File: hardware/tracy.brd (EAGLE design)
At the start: 58.5 x 38 mm, 78 parts, among them IC1 SIM900, J1 U.FL, J2 U.FL, Q4 si2305cd, T1 BC846, T2 BC846, U1 SPX5205 3v3, U2 3339, U3 TC1014 2V8, X1 MOLEX_6VERTICAL, X2 MOLEX_2HORIZONTAL, Y1 32768Hz CFPX-217 12.5pF

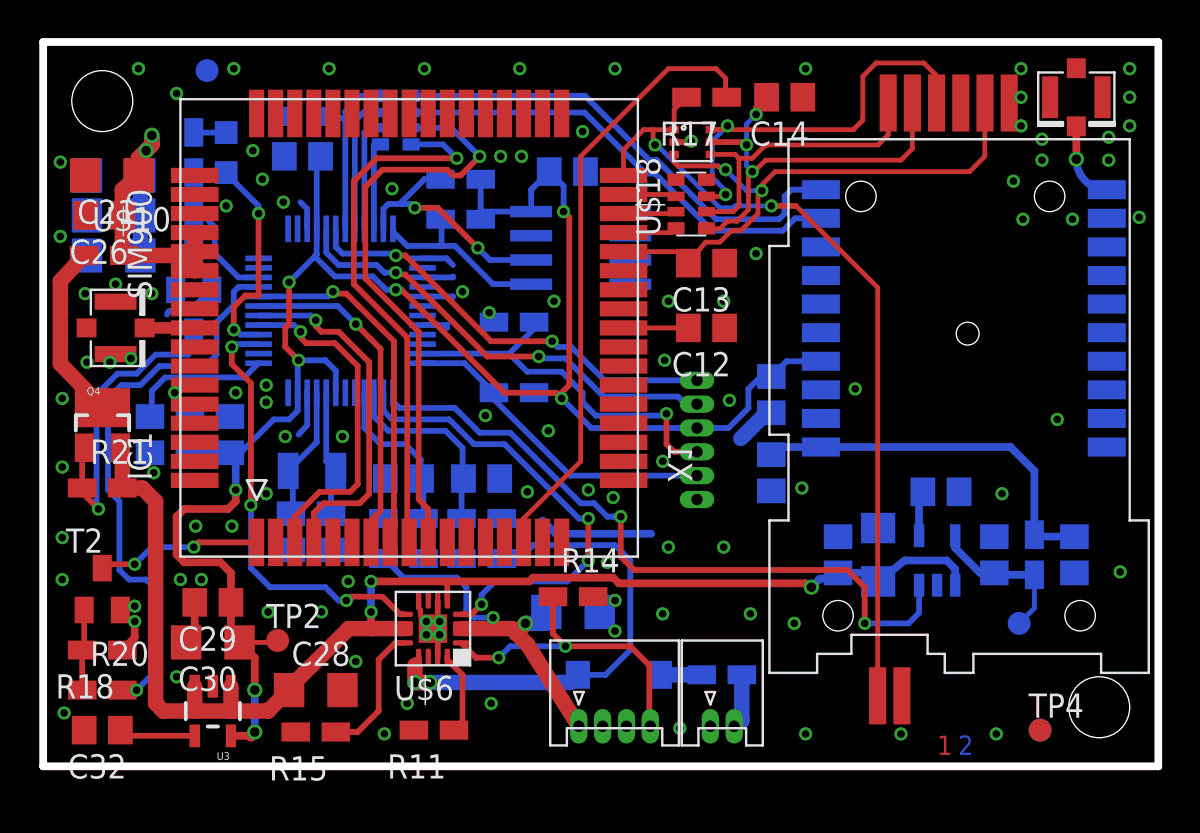
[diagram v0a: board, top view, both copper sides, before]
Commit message: rev 2
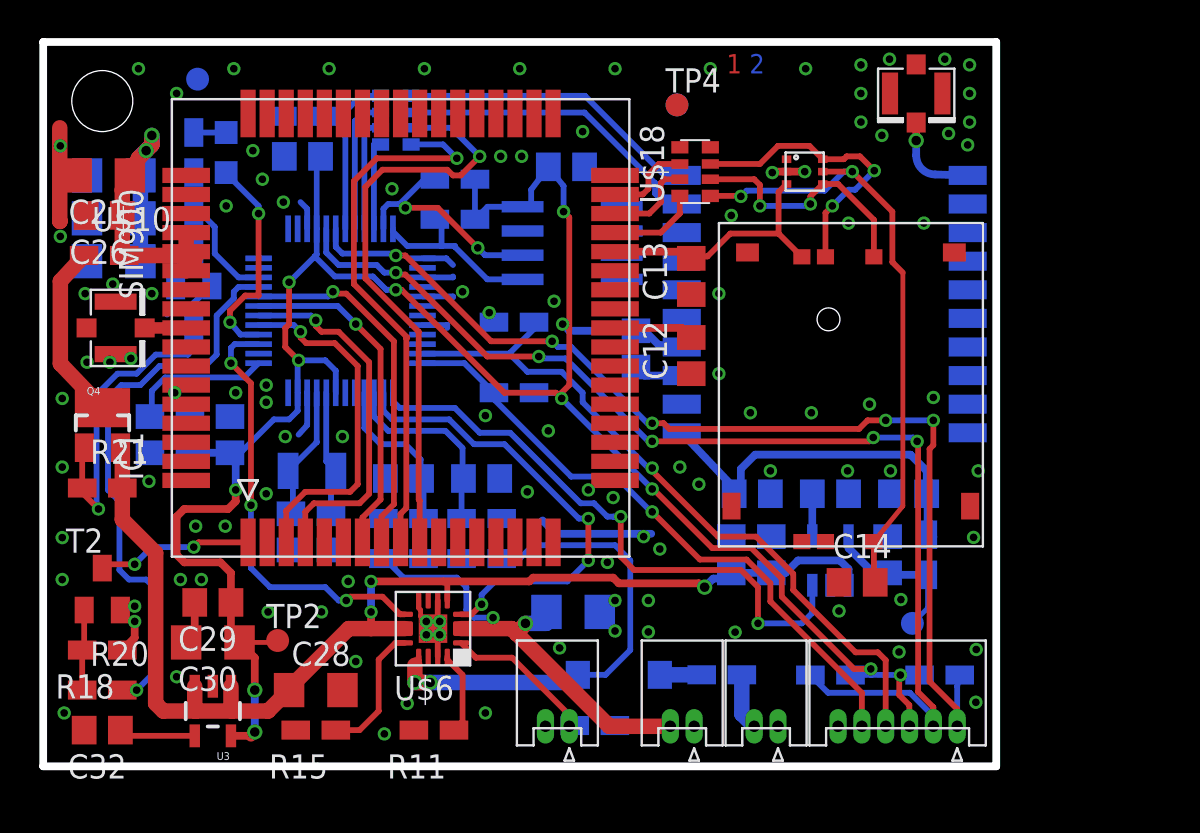
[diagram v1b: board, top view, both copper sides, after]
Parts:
- removed R17: 10k, rcl:R0805W
- removed U$19: LiPo, Simplex-Connectors:0530480401
- added R7, R8: 4k7, rcl:R0805W
- added X3: MOLEX_6HORIZONTAL, Simplex-Connectors:0530480610
- added X4: MOLEX_2HORIZONTAL, Simplex-Connectors:0530480210
- C11: value 10uF -> 1uF
- C3: device rcl:C1206 -> rcl:C0805
- U$3: value SIMLOCKC707_10M006_000_2 -> SIM_MOLEX_7880-0001; device Simplex-Connectors:SIMLOCK_C707_10M006 -> Simplex-Connectors:MOLEX_7880-0001
- X1: value MOLEX_6VERTICAL -> MOLEX_2HORIZONTAL; device Simplex-Connectors:0530470610 -> Simplex-Connectors:0530480210
- moved TP4 37.9 mm to (33.2, 34.7)
- moved TP6 37.9 mm to (33.2, 34.7)
- moved U$3 28.0 mm to (35.5, 28.5), turned to 270 degrees
- moved U$7 26.3 mm to (40.9, 34.5)
- moved C14 25.7 mm to (42.7, 9.65), turned to 0 degrees
- moved X1 12.6 mm to (38.5, 2.10), flipped to the top, turned to 180 degrees
- moved C5 9.27 mm to (45.4, 14.3), turned to 0 degrees
- moved J1 8.40 mm to (45.8, 35.3)
- moved C3 7.70 mm to (36.1, 11.1)
- moved C11 7.49 mm to (31.1, 21.9)
- moved U2 7.34 mm to (33.0, 32.2)
- moved R14 6.86 mm to (28.9, 2.14), flipped to the bottom, turned to 180 degrees
- moved U$8 6.10 mm to (39.0, 30.6)
- moved C4 5.80 mm to (41.3, 14.3)
- moved C1 5.60 mm to (44.3, 11.1)
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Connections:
- removed net N$42: IC1.34, R17.2, U$3.LOCK_1, U$8.1
- removed net N$43: IC1.15, R17.1
- net 2V8: now also R7.1, R8.1, X3.3; no longer X1.4
- net 5V: now also X1.2; no longer X2.2
- net BAT: now also X2.2; no longer U$19.1
- net GND: now also U$3.SH@1, U$3.SH@2, U$3.SH@3, U$3.SH@4, X3.6, X4.2; no longer U$19.2, U$19.3, U$3.LOCK_2
- net P4.0: now also R8.2, X3.2; no longer X1.5
- net P4.1: now also R7.2, X3.1; no longer X1.6
- net RST: now also X3.5; no longer X1.2
- net TEST: now also X3.4; no longer X1.3
- net TS: now also X4.1; no longer U$19.4
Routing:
- net N$42: track 43.5 -> 0.00 mm, vias 2 -> 0
- net P4.0: track 24.0 -> 59.7 mm, vias 2 -> 5
- net P4.1: track 22.8 -> 55.9 mm, vias 2 -> 5
- net N$43: track 32.2 -> 0.00 mm
- net 2V8: track 102.6 -> 123.0 mm, vias 8 -> 12
- net SIM_VCC: track 31.3 -> 13.8 mm, vias 2 -> 0
- net TEST: track 20.0 -> 37.5 mm
- net RST: track 17.0 -> 32.7 mm, vias 0 -> 1
- net SIMLOCK_IO: track 22.7 -> 32.7 mm, vias 3 -> 2
- net GPS_RX: track 25.4 -> 15.9 mm
- net TS: track 17.0 -> 8.43 mm, vias 2 -> 0
- net GPS_TX: track 24.3 -> 16.6 mm
- net SIMLOCK_RST: track 22.6 -> 15.4 mm
- net GND: track 33.0 -> 39.4 mm, vias 101 -> 107
- net VIN: track 68.9 -> 63.0 mm
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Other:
- board size 58.5 x 38 mm -> 50 x 38 mm
- board text added: "10KOhm ts"
- board text added: "3.7V bat"
- board text removed: "bat"
